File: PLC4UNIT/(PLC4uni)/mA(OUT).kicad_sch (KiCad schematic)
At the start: 18 parts, among them T2 IRF9310TRPBF

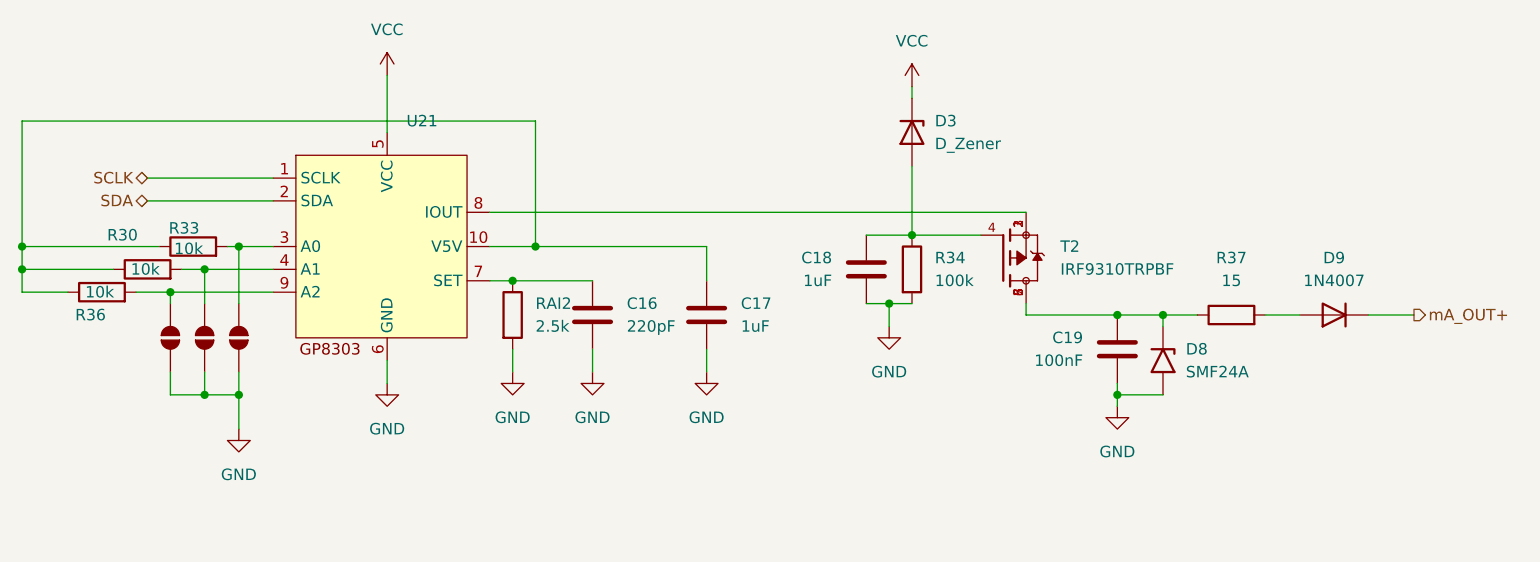
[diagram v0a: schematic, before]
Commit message: USB
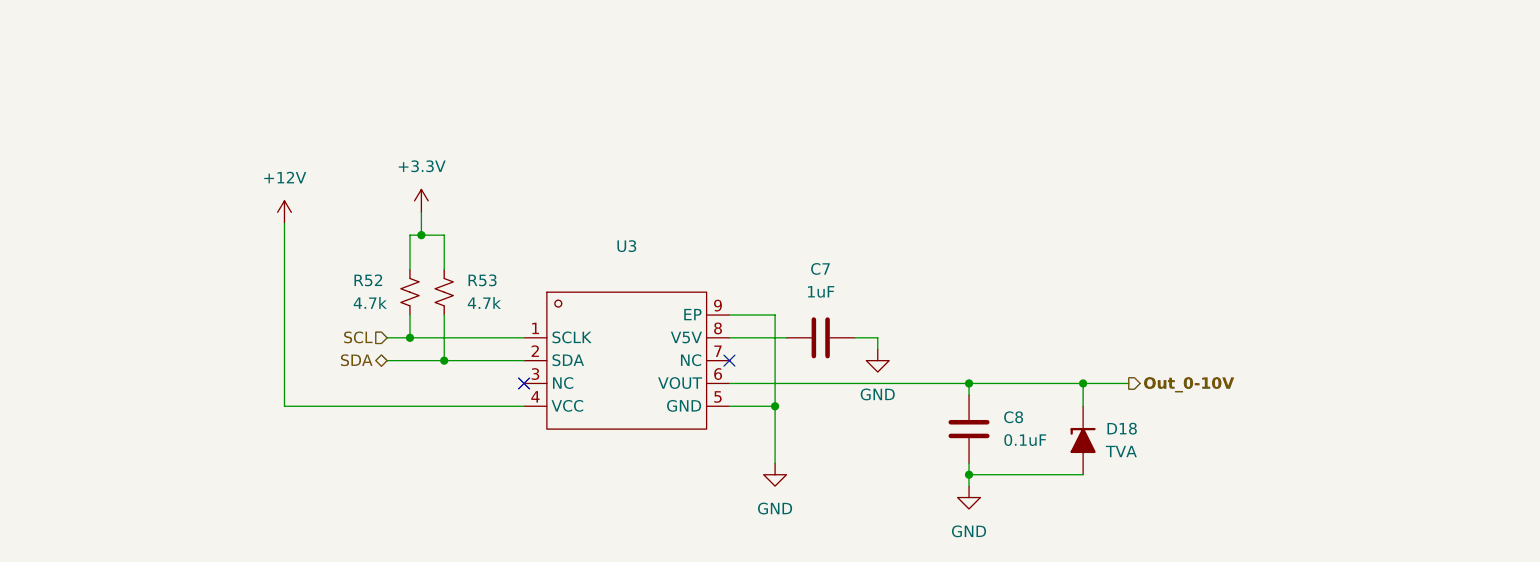
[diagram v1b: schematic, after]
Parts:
- removed C16: 220pF, Capacitor_SMD:C_0805_2012Metric, symbol Device:C
- removed C17, C18: 1uF, Capacitor_SMD:C_0805_2012Metric, symbol Device:C
- removed C19: 100nF, Capacitor_SMD:C_0805_2012Metric, symbol Device:C
- removed D3: D_Zener, Diode_SMD:D_0603_1608Metric, symbol Device:D_Zener
- removed D8: SMF24A, Diode_SMD:D_SMF, symbol Diode:SMF24A
- removed D9: 1N4007, Diode_SMD:D_0603_1608Metric_Pad1.05x0.95mm_HandSolder, symbol Diode:1N4007
- removed JP4, JP5, JP6: SolderJumper_2_Open, Jumper:SolderJumper-2_P1.3mm_Open_TrianglePad1.0x1.5mm, symbol Jumper:SolderJumper_2_Open
- removed R30, R33, R36: 10k, Resistor_SMD:R_0201_0603Metric, symbol Device:R
- removed R34: 100k, Resistor_SMD:R_0201_0603Metric, symbol Device:R
- removed R37: 15, Resistor_SMD:R_0201_0603Metric, symbol Device:R
- removed RAI2: 2.5k, Resistor_SMD:R_0201_0603Metric, symbol Device:R
- removed T2: IRF9310TRPBF, Package_SO:SOIC-8_5.3x5.3mm_P1.27mm, symbol Riqi_Parts:IRF9310TRPBF
- removed U21: ~, Package_SO:SSOP-10-1EP_3.9x4.9mm_P1mm_EP2.1x3.3mm, symbol Riqi_Parts:GP8303
- added C7: 1uF, PCM_Capacitor_SMD_AKL:C_0603_1608Metric, symbol PCM_Capacitor_US_AKL:C_0603
- added C8: 0.1uF, PCM_Capacitor_SMD_AKL:C_0603_1608Metric, symbol PCM_Capacitor_US_AKL:C_0603
- added D18: TVA, PCM_Diode_SMD_AKL:D_SOD-123F, symbol PCM_Diode_TVS_AKL:SMF12A
- added R52, R53: 4.7k, PCM_SparkFun-Resistor:R_0603_1608Metric, symbol PCM_SparkFun-Resistor:4.7k_0603
- added U3: ~, Lib_GP8211S-TC50-EW:ESOP-8_L4.9-W3.9-P1.27-LS6.0-BL-EP, symbol GP8211S-TC50-EW:root_0_GP8211S-TC50-EW_
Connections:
- net GND: now also C7.2, C8.1, D18.2 (A), U3.5 (GND), U3.9 (EP)
- net SDA: now also R53.2, U3.2 (SDA)
- new net: C7.1, U3.8 (V5V)
- new net +12V: U3.4 (VCC)
- new net +3.3V: R52.2, R53.1
- new net Out_0-10V: C8.2, D18.1 (K), U3.6 (VOUT)
- new net SCL: R52.1, U3.1 (SCLK)
- no-connect marks 0 -> 2
